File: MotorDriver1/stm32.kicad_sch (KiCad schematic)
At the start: 31 parts, among them IC1 STM32C092RCT6, IC2 TPS22916CNYFPR, J1 GT-USB-7010ASV, SW1 K2-6639SP-C4SC-04, SW2 K2-6639SP-C4SC-04, SW3 K2-6639SP-C4SC-04, U1 CH340X, Y1 48 MHz, Y2 32.768 kHz

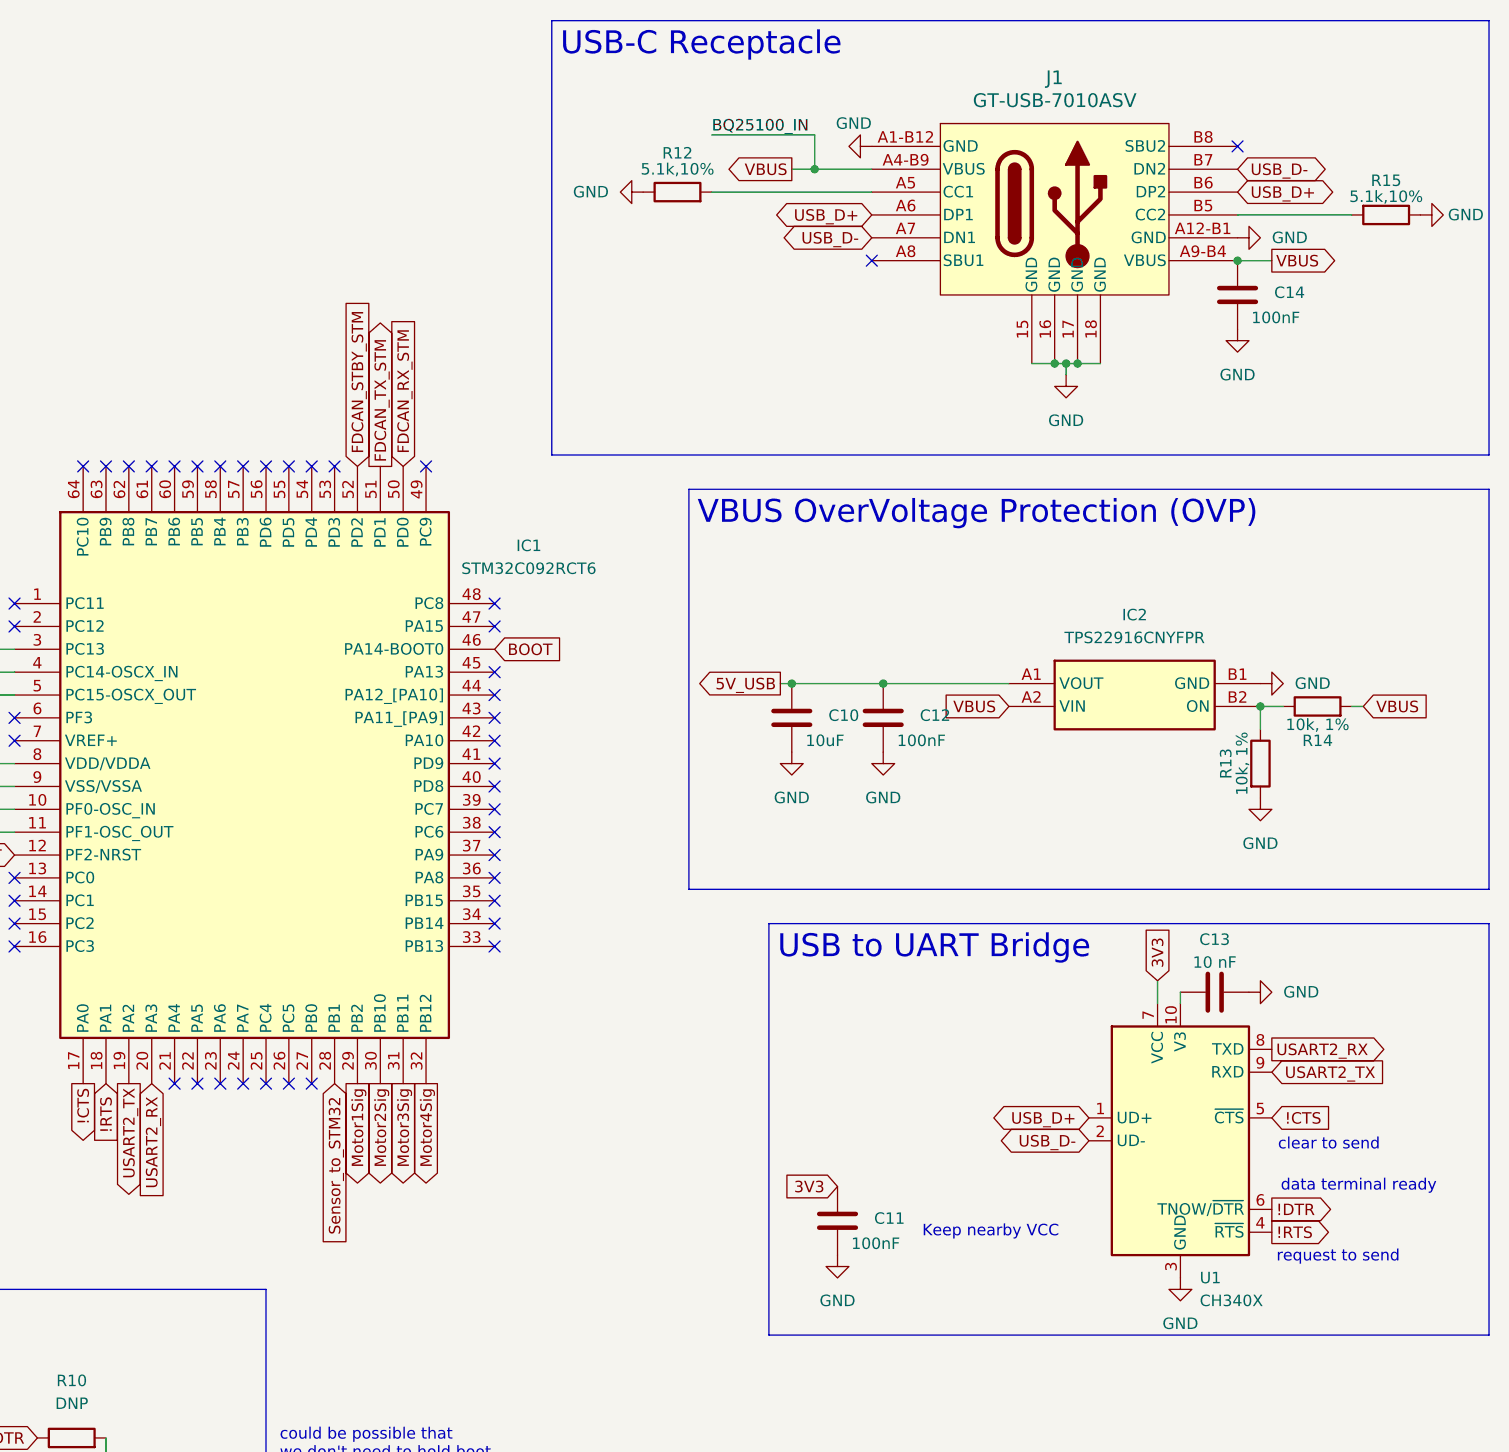
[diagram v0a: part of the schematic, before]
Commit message: laid out PCB
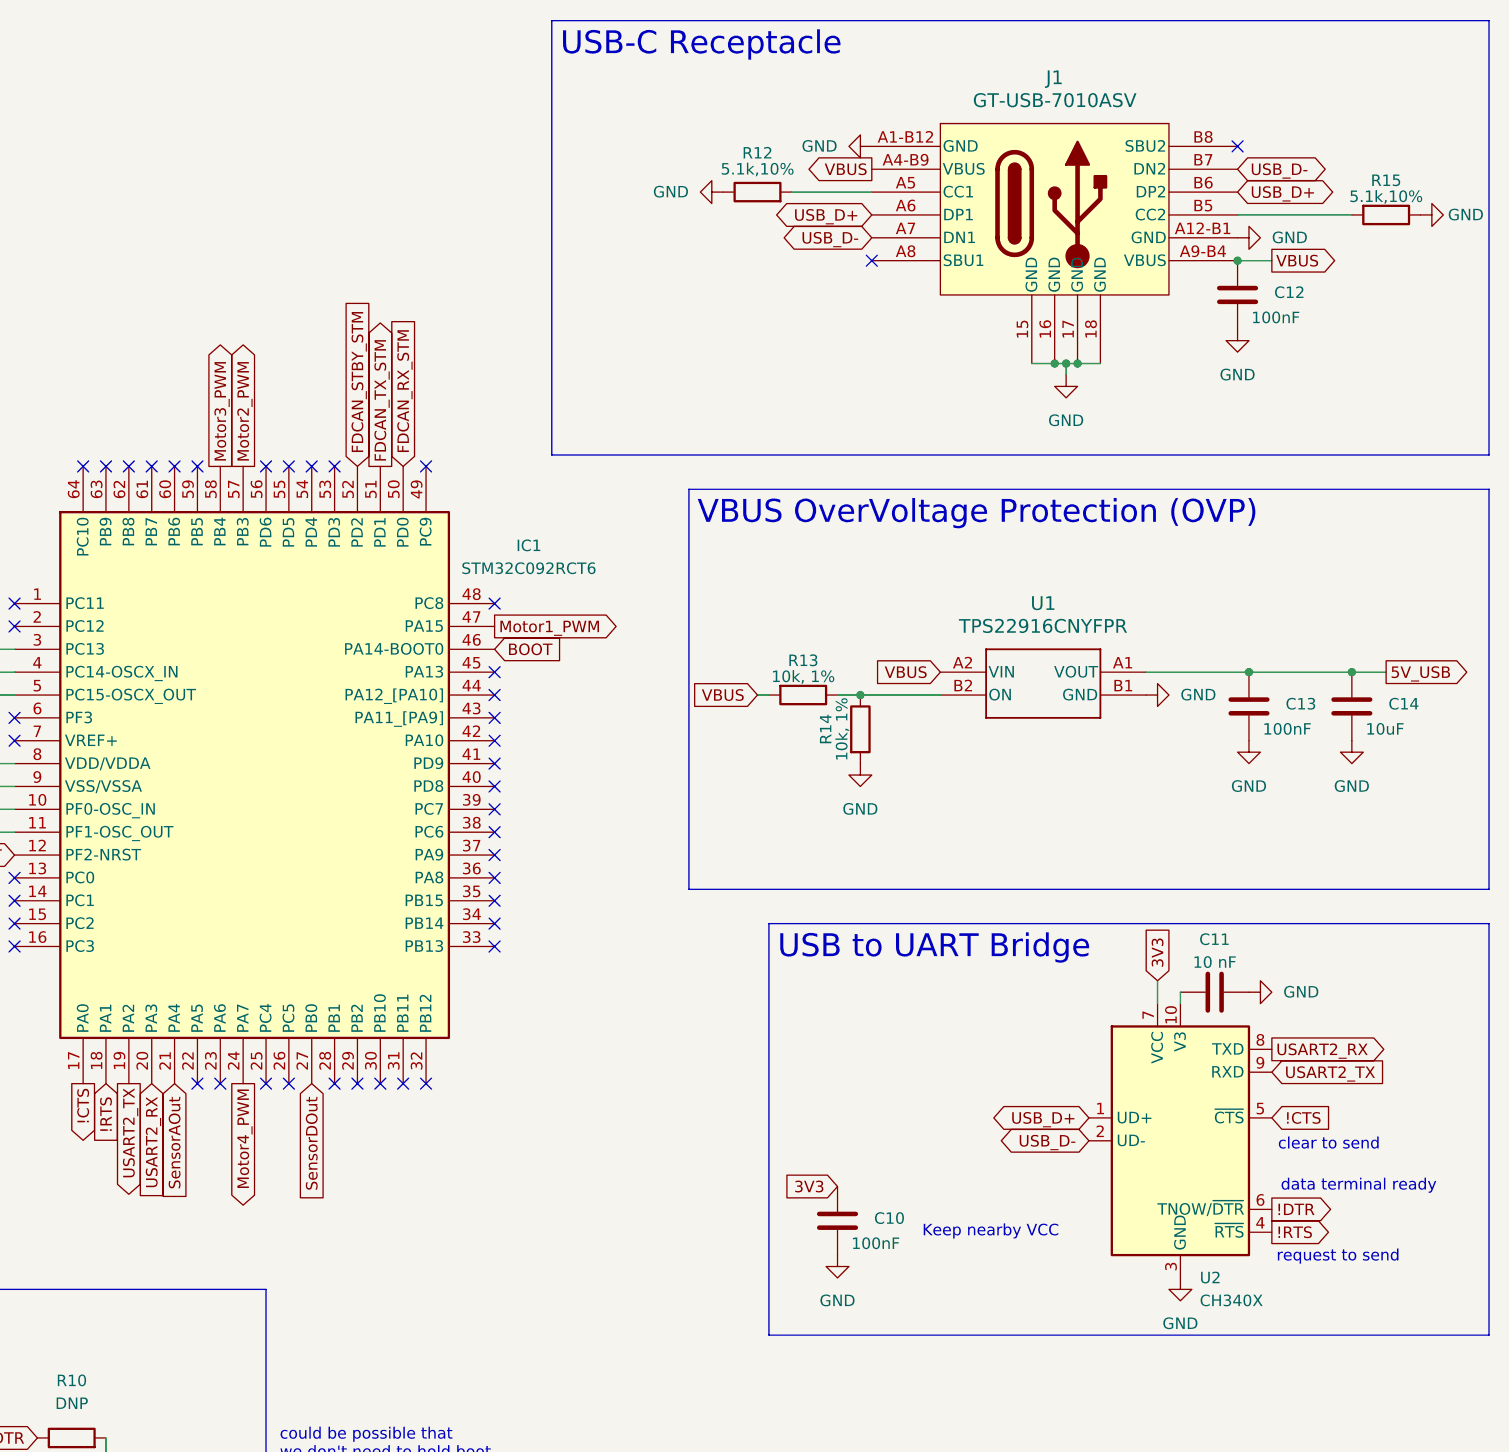
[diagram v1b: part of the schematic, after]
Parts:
- removed C10: 10uF, Capacitor_SMD:C_1206_3216Metric, symbol Device:C
- removed C12: 100nF, Capacitor_SMD:C_0402_1005Metric, symbol Device:C
- removed IC2: TPS22916CNYFPR, footprintLib:BGA6N40P3X2_157X88X50N, symbol pcb:TPS22916CNYFPR
- added C13: 100nF, Capacitor_SMD:C_0402_1005Metric, symbol Device:C
- added C14: 10uF, Capacitor_SMD:C_1206_3216Metric, symbol Device:C
- added U1: TPS22916CNYFPR, footprintLib:TPS22916CNYFPR, symbol pcb:TPS22916CNYFPR
- SW1, SW2, SW3: footprint Button_Switch_SMD:SW_Push_1P1T_NO_CK_KSC6xxJ -> footprintLib:K2-6639SP-C4SC-04
- renumbered C11 to C10, C13 to C11, C14 to C12, U1 to U2
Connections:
- net 5V_USB: now also C13.2, C14.2, U1.A1 (VOUT)
- net GND: now also R14.2, C13.1, C14.1, U1.B1 (GND); no longer R13.2
- net VBUS: now also R13.2, U1.A2 (VIN); no longer R14.2
- net at R13.1, R14.1: now also U1.B2 (ON)
- net SensorAOut: now reaches IC1.21 (PA4)
- net Motor4_PWM: now reaches IC1.24 (PA7)
- net SensorDOut: now reaches IC1.27 (PB0)
- net Motor1_PWM: now reaches IC1.47 (PA15)
- net Motor2_PWM: now reaches IC1.57 (PB3)
- net Motor3_PWM: now reaches IC1.58 (PB4)
- net Motor1Sig: no longer names the net of IC1.29 (PB2)
- net Motor2Sig: no longer names the net of IC1.30 (PB10)
- net Motor3Sig: no longer names the net of IC1.31 (PB11)
- net Motor4Sig: no longer names the net of IC1.32 (PB12)
- net Sensor_to_STM32: no longer names the net of IC1.28 (PB1)
- no-connect marks 46 -> 45
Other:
- moved on the sheet: R12
